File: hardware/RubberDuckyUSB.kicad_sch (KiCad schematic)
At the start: 10 parts, among them J1 USB_A, J2 USB_A, J3 Conn_01x04_Pin, J4 Conn_02x03_Odd_Even, J5 Conn_01x04_Pin, U1 ATTINY85-20SU

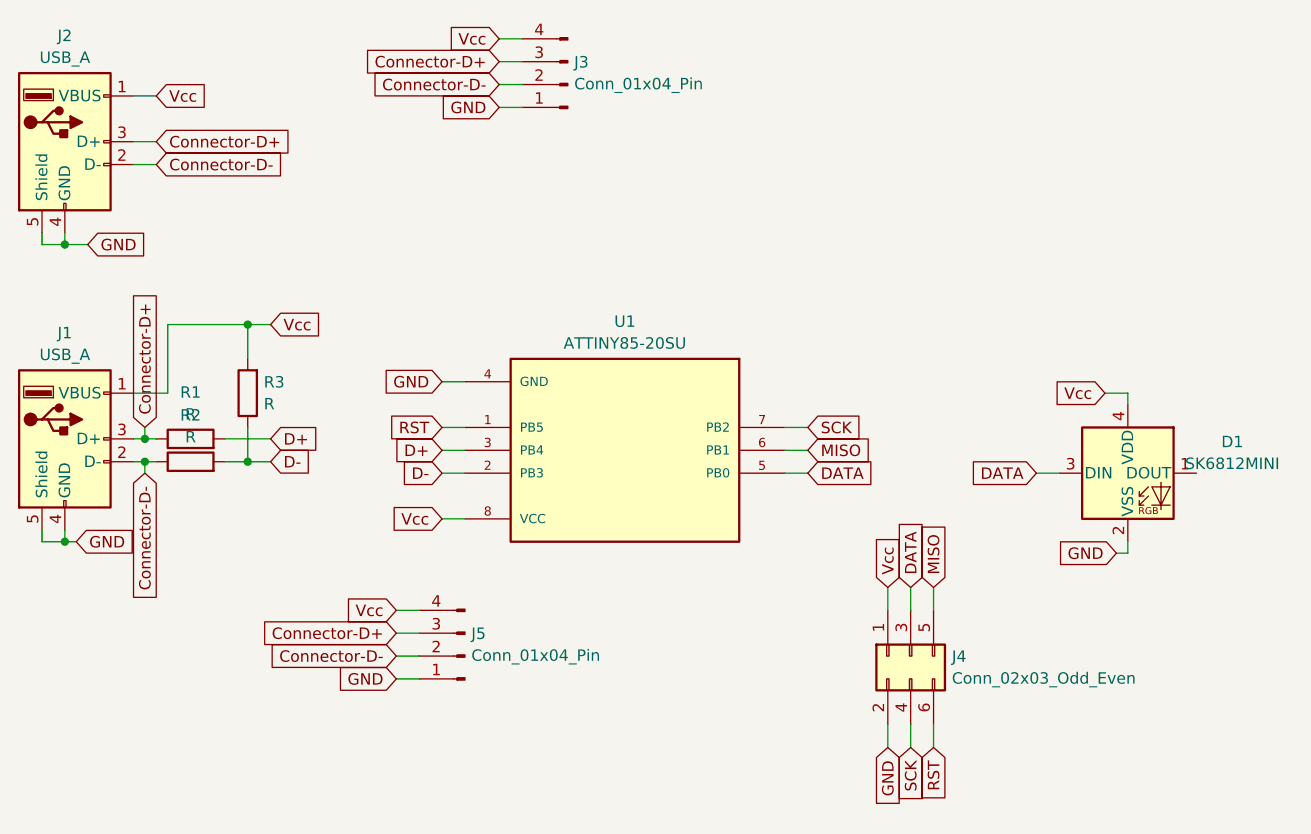
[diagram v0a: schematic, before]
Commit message: Revising hardware files
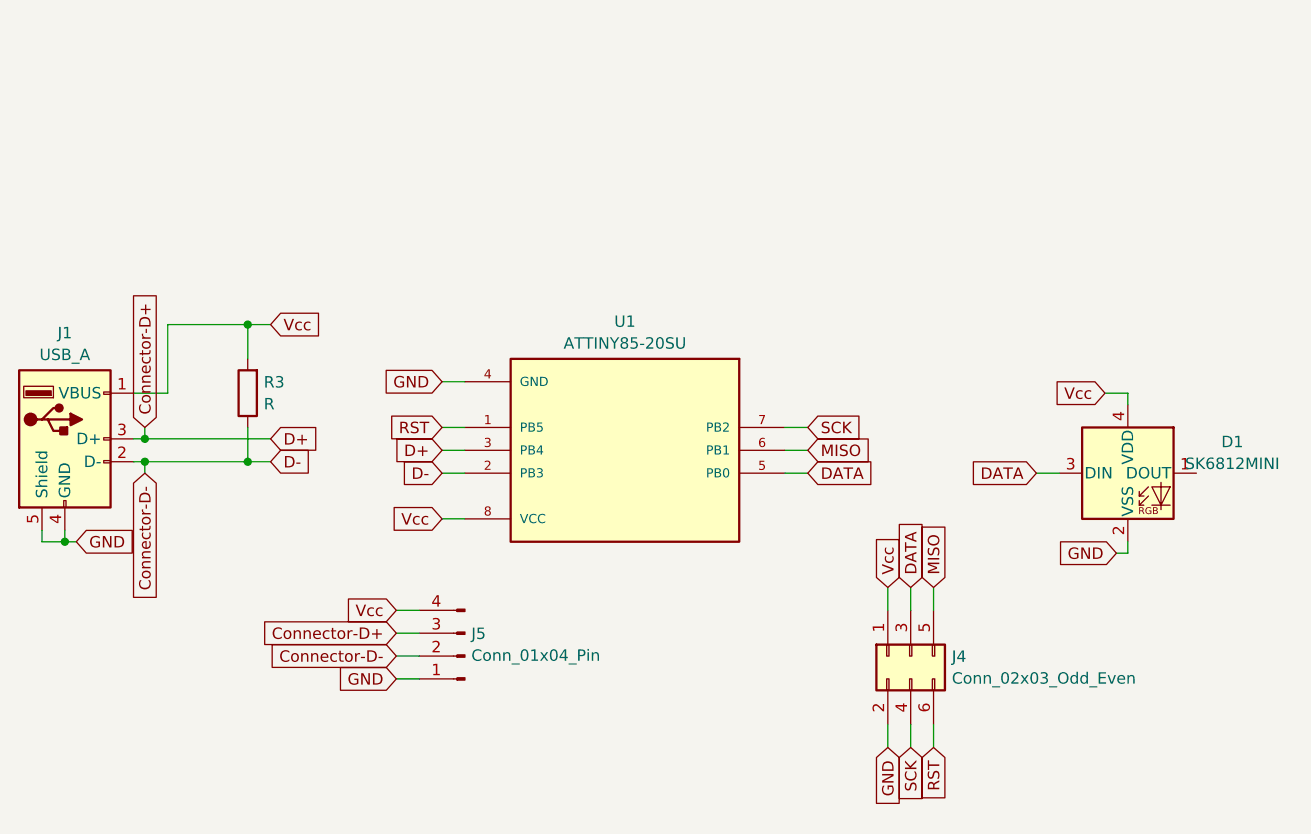
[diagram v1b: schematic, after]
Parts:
- removed J2: USB_A, Connectors:usb-PCB, symbol Connector:USB_A
- removed J3: Conn_01x04_Pin, Connector_PinHeader_2.54mm:PinHeader_1x04_P2.54mm_Vertical, symbol Connector:Conn_01x04_Pin
- removed R1, R2: R, Resistor_SMD:R_0805_2012Metric_Pad1.20x1.40mm_HandSolder, symbol Device:R
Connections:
- net D+ is gone; now on net Connector-D+: U1.3 (PB4)
- net D- is gone; now on net Connector-D-: R3.1, U1.2 (PB3)
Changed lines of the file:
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@@
 (kicad_sch (version 20230121) (generator eeschema)
   (paper "A4")
-  (junction (at 85.09 58.42) (diameter 0) (color 0 0 0 0)
-  )
   (junction (at 93.98 80.01) (diameter 0) (color 0 0 0 0)
   )
@@
     (stroke (width 0) (type default))
   )
-  (wire (pts (xy 82.55 58.42) (xy 85.09 58.42))
-    (stroke (width 0) (type default))
-  )
-  (wire (pts (xy 133.35 35.56) (xy 135.89 35.56))
-    (stroke (width 0) (type default))
-  )
   (wire (pts (xy 85.09 90.17) (xy 85.09 91.44))
     (stroke (width 0) (type default))
   )
-  (wire (pts (xy 82.55 57.15) (xy 82.55 58.42))
-    (stroke (width 0) (type default))
-  )
   (wire (pts (xy 96.52 67.31) (xy 105.41 67.31))
     (stroke (width 0) (type default))
@@
     (stroke (width 0) (type default))
   )
-  (wire (pts (xy 92.71 49.53) (xy 95.25 49.53))
-    (stroke (width 0) (type default))
-  )
   (wire (pts (xy 82.55 90.17) (xy 82.55 91.44))
     (stroke (width 0) (type default))
@@
     (stroke (width 0) (type default))
   )
-  (wire (pts (xy 102.87 80.01) (xy 107.95 80.01))
+  (wire (pts (xy 93.98 80.01) (xy 107.95 80.01))
     (stroke (width 0) (type default))
   )
@@
     (stroke (width 0) (type default))
   )
-  (wire (pts (xy 85.09 57.15) (xy 85.09 58.42))
-    (stroke (width 0) (type default))
-  )
   (wire (pts (xy 200.66 74.93) (xy 203.2 74.93))
     (stroke (width 0) (type default))
@@
     (stroke (width 0) (type default))
   )
-  (wire (pts (xy 93.98 82.55) (xy 95.25 82.55))
+  (wire (pts (xy 93.98 82.55) (xy 105.41 82.55))
     (stroke (width 0) (type default))
   )
@@
     (stroke (width 0) (type default))
   )
-  (wire (pts (xy 133.35 43.18) (xy 135.89 43.18))
-    (stroke (width 0) (type default))
-  )
   (wire (pts (xy 176.53 96.52) (xy 176.53 99.06))
     (stroke (width 0) (type default))
   )
-  (wire (pts (xy 85.09 58.42) (xy 87.63 58.42))
-    (stroke (width 0) (type default))
-  )
   (wire (pts (xy 121.92 101.6) (xy 124.46 101.6))
     (stroke (width 0) (type default))
@@
     (stroke (width 0) (type default))
   )
-  (wire (pts (xy 133.35 40.64) (xy 135.89 40.64))
-    (stroke (width 0) (type default))
-  )
   (wire (pts (xy 193.04 83.82) (xy 195.58 83.82))
     (stroke (width 0) (type default))
@@
     (stroke (width 0) (type default))
   )
-  (wire (pts (xy 92.71 46.99) (xy 95.25 46.99))
-    (stroke (width 0) (type default))
-  )
   (wire (pts (xy 85.09 91.44) (xy 86.36 91.44))
     (stroke (width 0) (type default))
   )
-  (wire (pts (xy 133.35 38.1) (xy 135.89 38.1))
-    (stroke (width 0) (type default))
-  )
   (wire (pts (xy 165.1 78.74) (xy 167.64 78.74))
     (stroke (width 0) (type default))
@@
     (stroke (width 0) (type default))
   )
-  (wire (pts (xy 102.87 82.55) (xy 105.41 82.55))
-    (stroke (width 0) (type default))
-  )
   (wire (pts (xy 93.98 82.55) (xy 93.98 83.82))
     (stroke (width 0) (type default))
@@
     (stroke (width 0) (type default))
   )
-  (wire (pts (xy 93.98 80.01) (xy 95.25 80.01))
-    (stroke (width 0) (type default))
-  )
   (wire (pts (xy 179.07 111.76) (xy 179.07 114.3))
     (stroke (width 0) (type default))
@@
     (stroke (width 0) (type default))
   )
-  (wire (pts (xy 92.71 41.91) (xy 95.25 41.91))
-    (stroke (width 0) (type default))
-  )
   (global_label "MISO" (shape input) (at 181.61 96.52 90) (fields_autoplaced)
     (effects (font (size 1.27 1.27)) (justify left))
@@
     )
   )
-  (global_label "Connector-D-" (shape input) (at 133.35 40.64 180) (fields_autoplaced)
-    (effects (font (size 1.27 1.27)) (justify right))
-    (property "Intersheetrefs" "${INTERSHEET_REFS}" (at 116.3949 40.64 0)
-      (effects (font (size 1.27 1.27)) (justify right) hide)
-    )
-  )
   (global_label "Connector-D-" (shape input) (at 121.92 104.14 180) (fields_autoplaced)
     (effects (font (size 1.27 1.27)) (justify right))
@@
     )
   )
-  (global_label "GND" (shape input) (at 133.35 43.18 180) (fields_autoplaced)
-    (effects (font (size 1.27 1.27)) (justify right))
-    (property "Intersheetrefs" "${INTERSHEET_REFS}" (at 126.4943 43.18 0)
-      (effects (font (size 1.27 1.27)) (justify right) hide)
-    )
-  )
-  (global_label "Vcc" (shape input) (at 133.35 35.56 180) (fields_autoplaced)
-    (effects (font (size 1.27 1.27)) (justify right))
-    (property "Intersheetrefs" "${INTERSHEET_REFS}" (at 127.099 35.56 0)
-      (effects (font (size 1.27 1.27)) (justify right) hide)
-    )
-  )
-  (global_label "GND" (shape input) (at 87.63 58.42 0) (fields_autoplaced)
-    (effects (font (size 1.27 1.27)) (justify left))
-    (property "Intersheetrefs" "${INTERSHEET_REFS}" (at 94.4857 58.42 0)
-      (effects (font (size 1.27 1.27)) (justify left) hide)
-    )
-  )
   (global_label "Connector-D+" (shape input) (at 93.98 78.74 90) (fields_autoplaced)
     (effects (font (size 1.27 1.27)) (justify left))
@@
     )
   )
-  (global_label "Connector-D-" (shape input) (at 95.25 49.53 0) (fields_autoplaced)
-    (effects (font (size 1.27 1.27)) (justify left))
-    (property "Intersheetrefs" "${INTERSHEET_REFS}" (at 112.2051 49.53 0)
-      (effects (font (size 1.27 1.27)) (justify left) hide)
-    )
-  )
   (global_label "SCK" (shape input) (at 167.64 78.74 0) (fields_autoplaced)
     (effects (font (size 1.27 1.27)) (justify left))
@@
     )
   )
-  (global_label "Connector-D+" (shape input) (at 95.25 46.99 0) (fields_autoplaced)
-    (effects (font (size 1.27 1.27)) (justify left))
-    (property "Intersheetrefs" "${INTERSHEET_REFS}" (at 112.2051 46.99 0)
-      (effects (font (size 1.27 1.27)) (justify left) hide)
-    )
-  )
   (global_label "Connector-D+" (shape input) (at 121.92 101.6 180) (fields_autoplaced)
     (effects (font (size 1.27 1.27)) (justify right))
@@
     )
   )
-  (global_label "Vcc" (shape input) (at 95.25 41.91 0) (fields_autoplaced)
-    (effects (font (size 1.27 1.27)) (justify left))
-    (property "Intersheetrefs" "${INTERSHEET_REFS}" (at 101.501 41.91 0)
-      (effects (font (size 1.27 1.27)) (justify left) hide)
-    )
-  )
   (global_label "GND" (shape input) (at 121.92 106.68 180) (fields_autoplaced)
     (effects (font (size 1.27 1.27)) (justify right))
@@
     (property "Intersheetrefs" "${INTERSHEET_REFS}" (at 93.2157 91.44 0)
       (effects (font (size 1.27 1.27)) (justify left) hide)
-    )
-  )
-  (global_label "Connector-D+" (shape input) (at 133.35 38.1 180) (fields_autoplaced)
-    (effects (font (size 1.27 1.27)) (justify right))
-    (property "Intersheetrefs" "${INTERSHEET_REFS}" (at 116.3949 38.1 0)
-      (effects (font (size 1.27 1.27)) (justify right) hide)
     )
   )
@@
     )
   )
-  (symbol (lib_id "Connector:USB_A") (at 85.09 46.99 0) (unit 1)
-    (in_bom yes) (on_board yes) (dnp no) (fields_autoplaced)
-    (property "Reference" "J2" (at 85.09 35.2257 0)
-      (effects (font (size 1.27 1.27)))
-    )
-    (property "Value" "USB_A" (at 85.09 37.6499 0)
-      (effects (font (size 1.27 1.27)))
-    )
-    (property "Footprint" "Connectors:usb-PCB" (at 88.9 48.26 0)
-      (effects (font (size 1.27 1.27)) hide)
-    )
-    (property "Datasheet" " ~" (at 88.9 48.26 0)
-      (effects (font (size 1.27 1.27)) hide)
-    )
-    (pin "1")
-    (pin "2")
-    (pin "3")
-    (pin "4")
-    (pin "5")
-    (instances
-      (project "RubberDuckyUSB"
-        (path "/8bf37dd3-a64d-4f1e-94bd-d70c0ea44f56"
-          (reference "J2") (unit 1)
-        )
-      )
-    )
-  )
-  (symbol (lib_id "Connector:Conn_01x04_Pin") (at 140.97 40.64 180) (unit 1)
-    (in_bom yes) (on_board yes) (dnp no) (fields_autoplaced)
-    (property "Reference" "J3" (at 141.6812 38.1579 0)
-      (effects (font (size 1.27 1.27)) (justify right))
-    )
-    (property "Value" "Conn_01x04_Pin" (at 141.6812 40.5821 0)
-      (effects (font (size 1.27 1.27)) (justify right))
-    )
-    (property "Footprint" "Connector_PinHeader_2.54mm:PinHeader_1x04_P2.54mm_Vertical" (at 140.97 40.64 0)
-      (effects (font (size 1.27 1.27)) hide)
-    )
-    (property "Datasheet" "~" (at 140.97 40.64 0)
-      (effects (font (size 1.27 1.27)) hide)
-    )
-    (pin "1")
-    (pin "2")
-    (pin "3")
-    (pin "4")
-    (instances
-      (project "RubberDuckyUSB"
-        (path "/8bf37dd3-a64d-4f1e-94bd-d70c0ea44f56"
-          (reference "J3") (unit 1)
-        )
-      )
-    )
-  )
   (symbol (lib_id "LED:SK6812MINI") (at 203.2 83.82 0) (unit 1)
     (in_bom yes) (on_board yes) (dnp no) (fields_autoplaced)
@@
         )
       )
-    )
-  )
-  (symbol (lib_id "Device:R") (at 99.06 82.55 90) (unit 1)
-    (in_bom yes) (on_board yes) (dnp no) (fields_autoplaced)
-    (property "Reference" "R2" (at 99.06 77.3897 90)
-      (effects (font (size 1.27 1.27)))
-    )
-    (property "Value" "R" (at 99.06 79.8139 90)
-      (effects (font (size 1.27 1.27)))
-    )
-    (property "Footprint" "Resistor_SMD:R_0805_2012Metric_Pad1.20x1.40mm_HandSolder" (at 99.06 84.328 90)
-      (effects (font (size 1.27 1.27)) hide)
-    )
-    (property "Datasheet" "~" (at 99.06 82.55 0)
-      (effects (font (size 1.27 1.27)) hide)
-    )
-    (pin "1")
-    (pin "2")
-    (instances
-      (project "RubberDuckyUSB"
-        (path "/8bf37dd3-a64d-4f1e-94bd-d70c0ea44f56"
-          (reference "R2") (unit 1)
-        )
-      )
-    )
-  )
-  (symbol (lib_id "Device:R") (at 99.06 80.01 90) (unit 1)
-    (in_bom yes) (on_board yes) (dnp no) (fields_autoplaced)
-    (property "Reference" "R1" (at 99.06 74.8497 90)
-      (effects (font (size 1.27 1.27)))
-    )
-    (property "Value" "R" (at 99.06 77.2739 90)
-      (effects (font (size 1.27 1.27)))
-    )
-    (property "Footprint" "Resistor_SMD:R_0805_2012Metric_Pad1.20x1.40mm_HandSolder" (at 99.06 81.788 90)
-      (effects (font (size 1.27 1.27)) hide)
-    )
-    (property "Datasheet" "~" (at 99.06 80.01 0)
-      (effects (font (size 1.27 1.27)) hide)
-    )
-    (pin "1")
-    (pin "2")
-    (instances
-      (project "RubberDuckyUSB"
-        (path "/8bf37dd3-a64d-4f1e-94bd-d70c0ea44f56"
-          (reference "R1") (unit 1)
-        )
-      )
